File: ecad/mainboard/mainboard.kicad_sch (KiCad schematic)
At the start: 58 parts, among them J1 TYPE-C-31-M-12, J2 SWD, J3 UART, SW1 TS-1187A-B-A-B, SW2 TS-1187A-B-A-B, SW3 SW_Push, SW4 SW_Push, U1 NCP1117ST33T3G, U2 USBLC6-2SC6, U2 W25Q128JVS, U3 RP2040, U4 74AHCT1G125, Y1 ABM8-272-T3

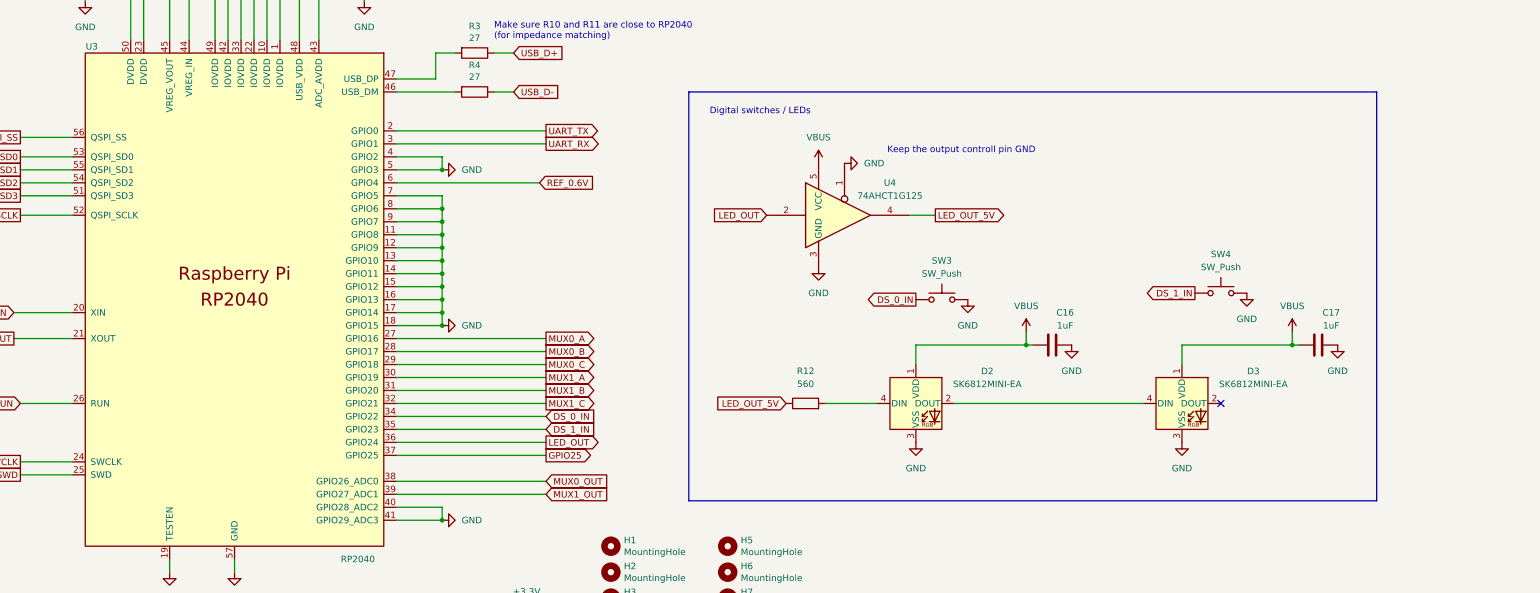
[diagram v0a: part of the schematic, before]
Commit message: prepare for the rev.1 board
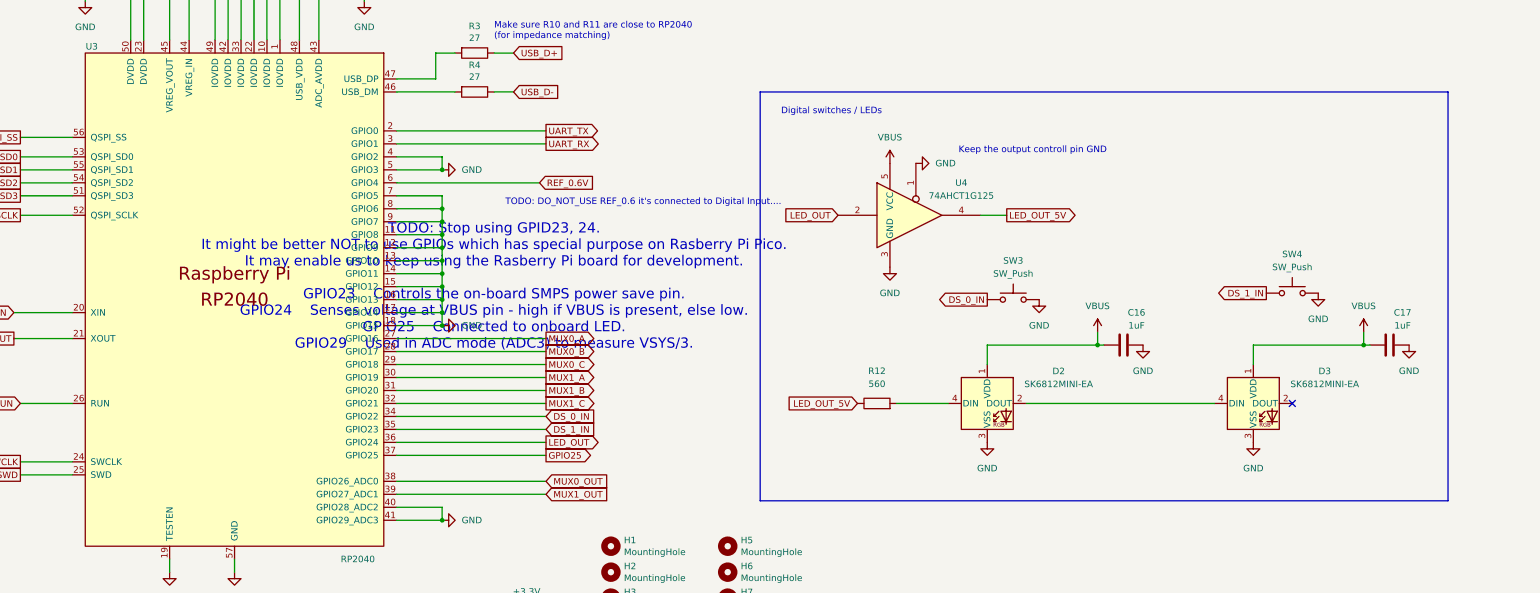
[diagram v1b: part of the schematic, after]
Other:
- note added: "TODO: DO_NOT_USE REF_0.6 it's connected to Digital Input...."
- note added: "TODO: Stop using GPID23, 24. It might be better NOT to use GPIOs which has special purpose on Rasberry Pi Pico. It may enable us to keep using the Rasberry Pi board for development. GPIO23 Controls the on-board SMPS power save pin. GPIO24 Senses voltage at VBUS pin - high if VBUS is present, else low. GPIO25 Connected to onboard LED. GPIO29 Used in ADC mode (ADC3) to measure VSYS/3."
- moved on the sheet: C16, C17, D2, D3, R12, SW3, SW4, U4
